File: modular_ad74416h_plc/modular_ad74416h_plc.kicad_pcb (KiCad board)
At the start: 2 copper layers, 5.1 x 5.1 mm, 1 part

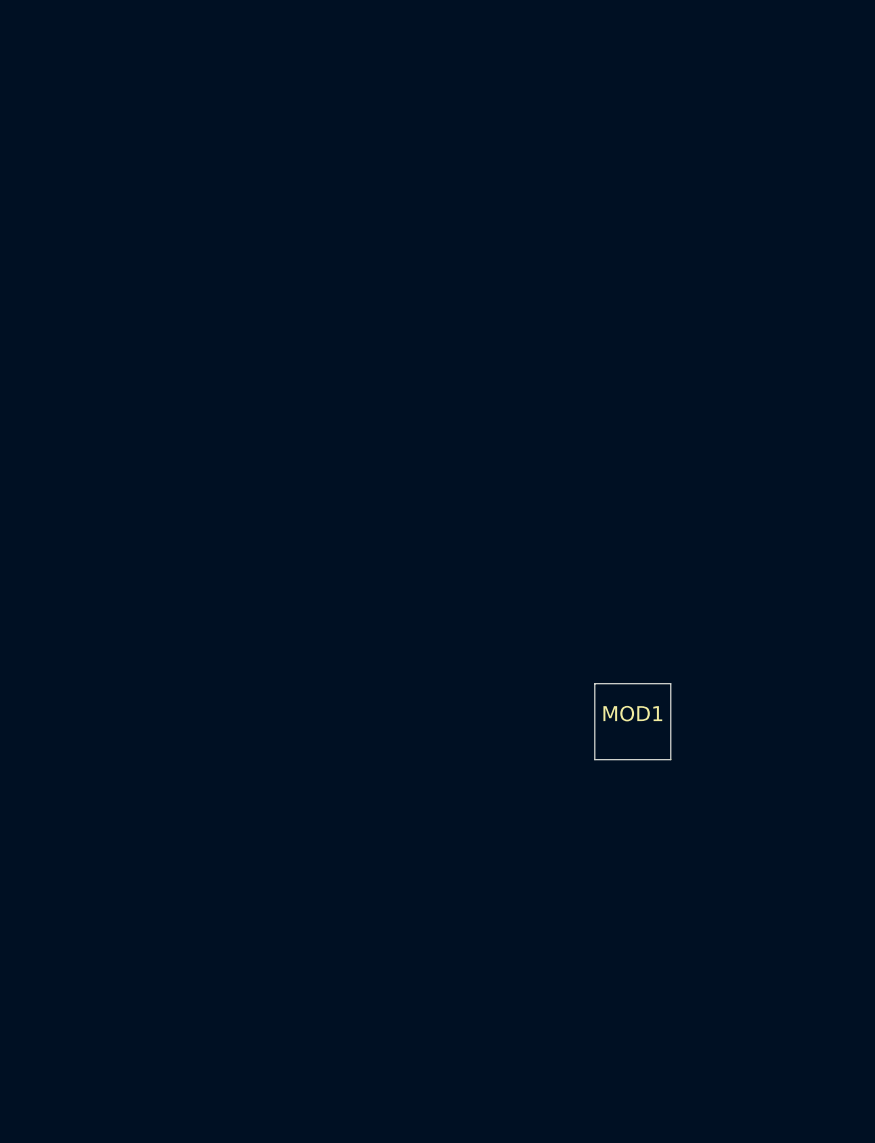
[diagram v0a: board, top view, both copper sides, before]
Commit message: backup
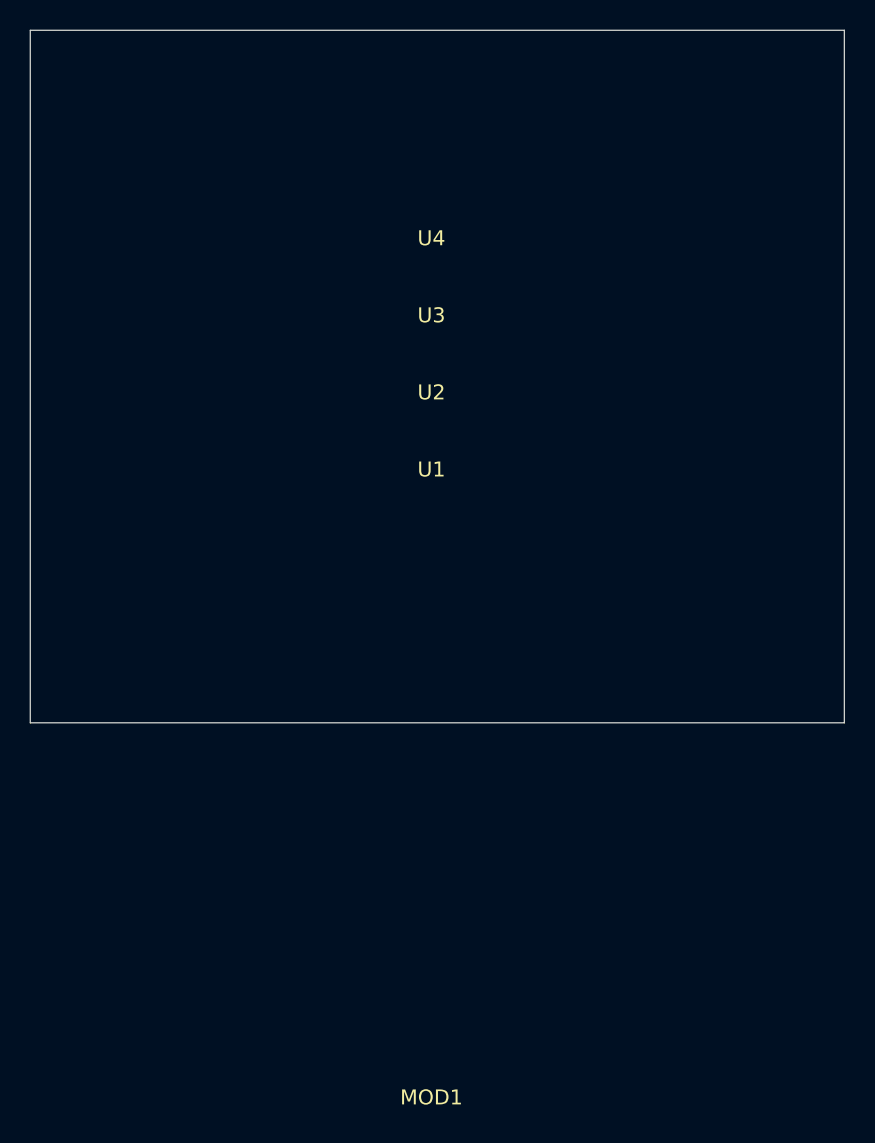
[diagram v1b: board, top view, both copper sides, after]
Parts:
- added U1: ~, modules_footprints:minimal_ad74416h, F.Cu at (143.0, 84.4)
- added U2: ~, modules_footprints:minimal_ad74416h, F.Cu at (143.0, 79.3)
- added U3: ~, modules_footprints:minimal_ad74416h, F.Cu at (143.0, 74.1)
- added U4: ~, modules_footprints:minimal_ad74416h, F.Cu at (143.0, 68.9)
- moved MOD1 28.9 mm to (143.0, 126.4)
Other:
- board size 5.1 x 5.1 mm -> 54.4 x 46.3 mm
